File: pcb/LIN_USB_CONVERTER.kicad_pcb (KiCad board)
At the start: 2 copper layers, 17.8 x 34 mm, 32 parts, among them J1 Conn_01x03, J2 Conn_01x03, J3 GS2, J4 USB_A, J5 Conn_01x02, P2 CONN_01X05, U1 TJA1028, U2 MAX12931, U3 MCP1700T-3302E/TT, U4 STM32F042G4U6

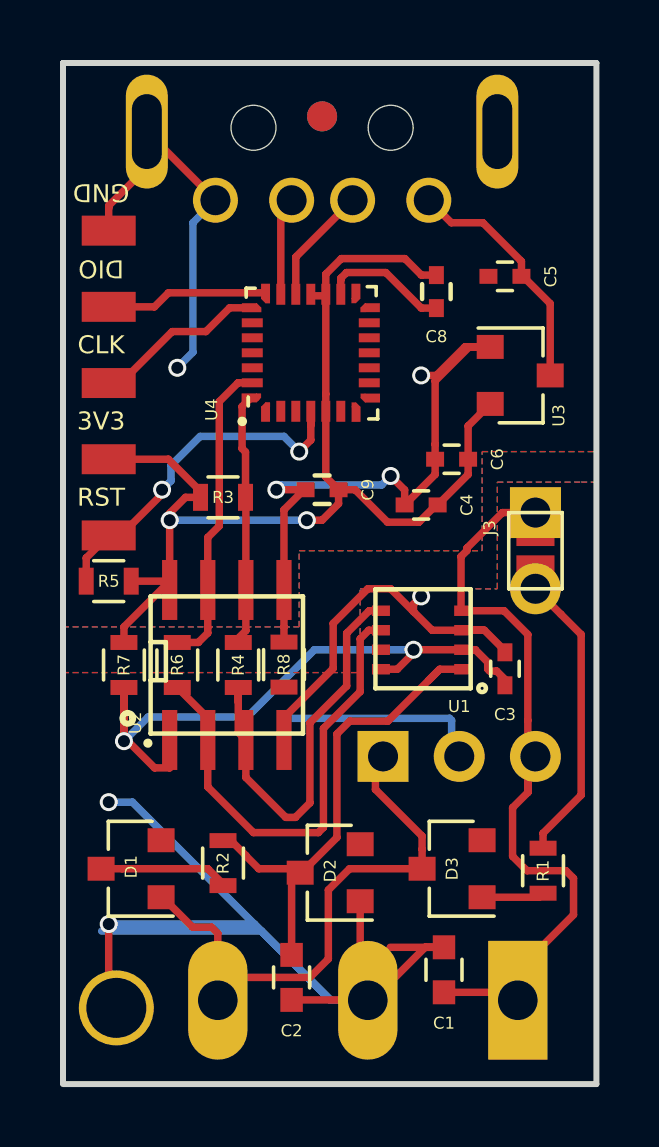
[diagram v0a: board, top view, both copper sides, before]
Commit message: PCB release
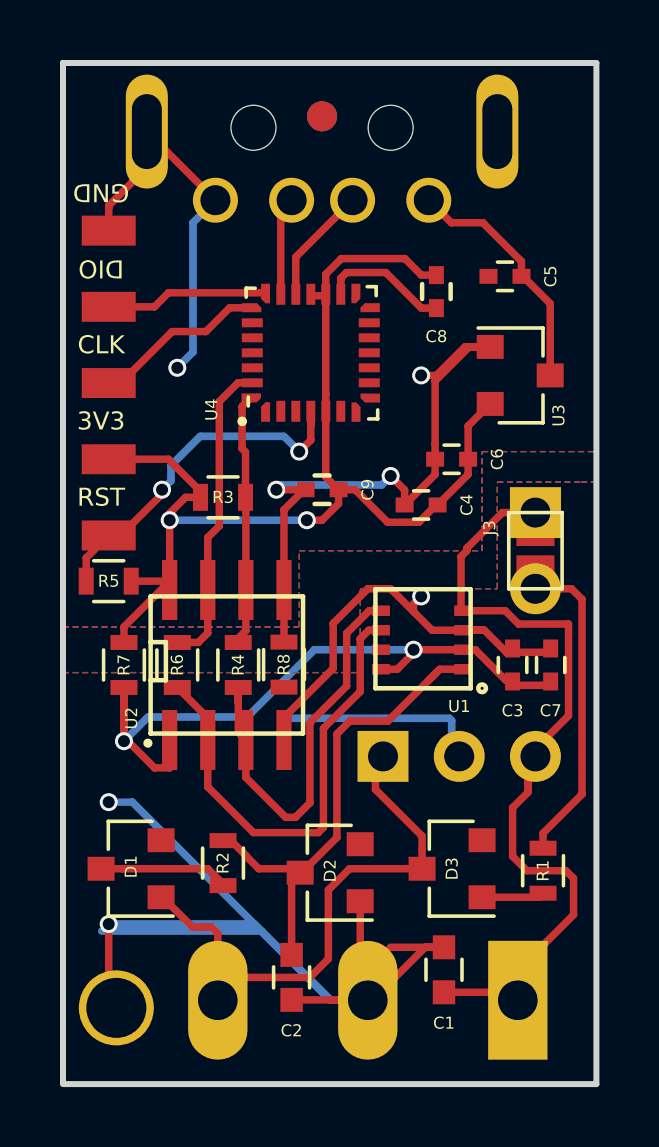
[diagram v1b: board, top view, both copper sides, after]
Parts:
- added C7: 10u, Capacitors_SMD:C_0402, F.Cu at (156.5, 98.4)
- J2: value Conn_01x03 -> TerminalBlock
- U1: value TJA1028 -> TJA1028TK/3V3/20/J
- U2: value MAX12931 -> MAX12931BASA+
- moved C3 0.28 mm to (155.2, 98.4)
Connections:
- U1 pad 7: Net-(U1-Pad7) -> (no net)
- U4 pad 10: Net-(U4-Pad10) -> (no net)
- U4 pad 11: Net-(U4-Pad11) -> (no net)
- U4 pad 12: Net-(U4-Pad12) -> (no net)
- U4 pad 13: Net-(U4-Pad13) -> (no net)
- U4 pad 2: Net-(U4-Pad2) -> (no net)
- U4 pad 23: Net-(U4-Pad23) -> (no net)
- U4 pad 24: Net-(U4-Pad24) -> (no net)
- U4 pad 25: Net-(U4-Pad25) -> (no net)
- U4 pad 26: Net-(U4-Pad26) -> (no net)
- U4 pad 3: Net-(U4-Pad3) -> (no net)
- U4 pad 6: Net-(U4-Pad6) -> (no net)
- U4 pad 9: Net-(U4-Pad9) -> (no net)
- mh1 pad 1: (no net) -> -BATT
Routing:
- net Net-(C1-Pad1): track 26.1 -> 28.3 mm
- net -BATT: track 62.7 -> 64.2 mm
- net +3.3VA: track 22.4 -> 23.7 mm
- net Net-(J3-Pad2): track 9.81 -> 10.5 mm
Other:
- board text added: "MASTER RESISTOR"

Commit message: PCB release
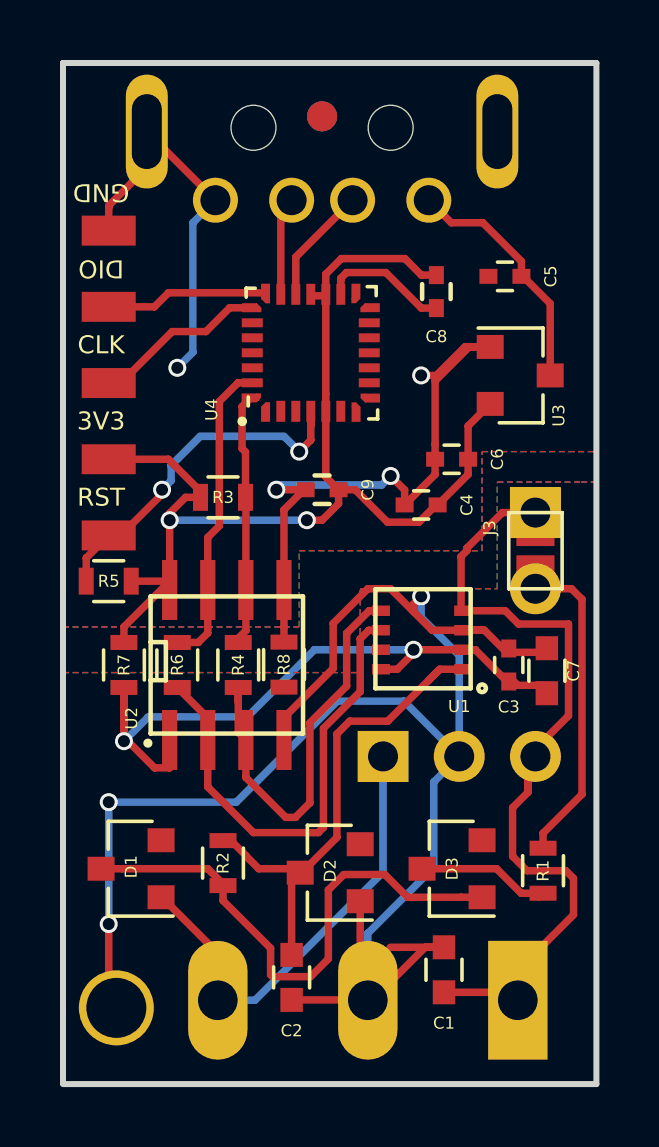
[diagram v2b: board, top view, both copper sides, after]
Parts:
- C7: footprint Capacitors_SMD:C_0402 -> Capacitors_SMD:C_0603
- moved C7 0.23 mm to (156.4, 98.6)
- moved C3 0.13 mm to (155.1, 98.4)
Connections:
- D1 pad 1: Net-(D1-Pad1) -> +BATT
- D1 pad 2: +BATT -> Net-(D1-Pad2)
- D3 pad 1: +BATT -> Net-(D3-Pad1)
- D3 pad 2: Net-(D3-Pad2) -> +BATT
- J1 pad 1: +BATT -> Net-(D1-Pad2)
- J2 pad 3: +BATT -> Net-(D1-Pad2)
- R1 pad 2: Net-(D3-Pad2) -> Net-(D3-Pad1)
- R2 pad 2: Net-(D1-Pad1) -> +BATT
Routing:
- net Net-(D1-Pad2): track 0.00 -> 18.4 mm
- net Net-(D3-Pad1): track 0.00 -> 4.56 mm
- net Net-(D1-Pad1): track 4.55 -> 0.00 mm
- net Net-(D3-Pad2): track 2.09 -> 0.00 mm
- net -BATT: track 64.2 -> 62.1 mm
- net +BATT: track 20.0 -> 18.3 mm
